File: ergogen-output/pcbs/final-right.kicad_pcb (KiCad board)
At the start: 2 copper layers, 161.7 x 120.6 mm, 61 parts

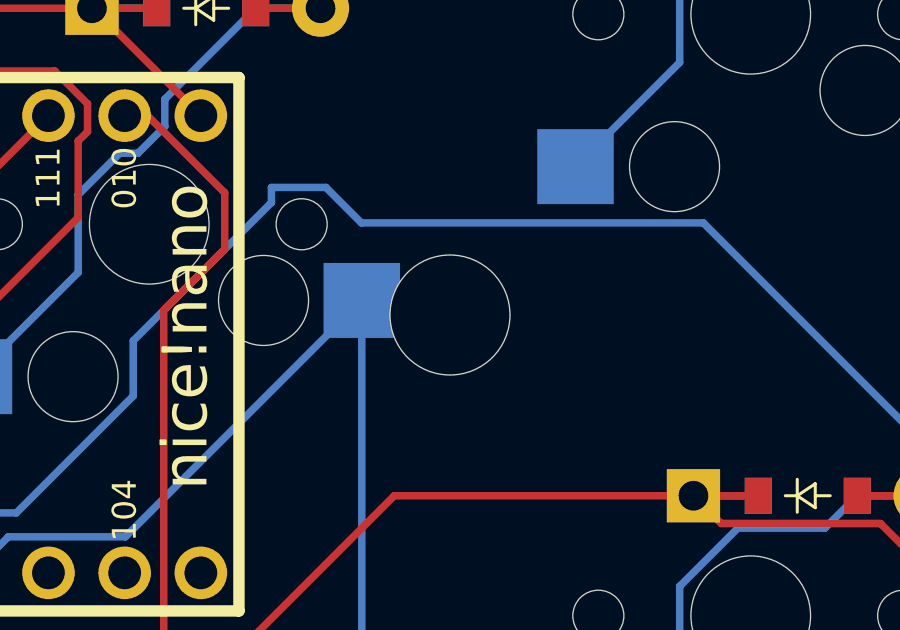
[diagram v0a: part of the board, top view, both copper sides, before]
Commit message: fix pcbs :(
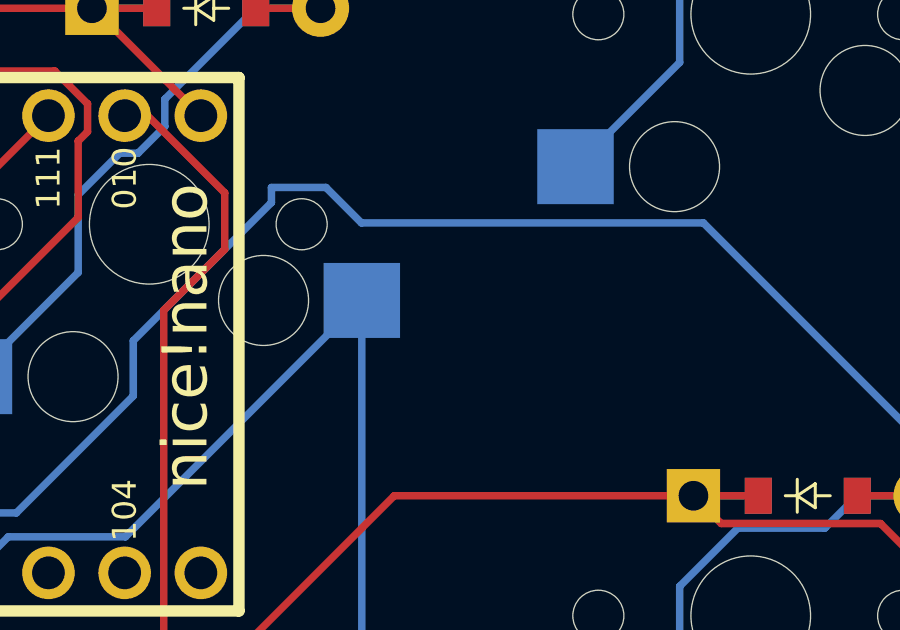
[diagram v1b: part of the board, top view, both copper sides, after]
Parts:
- removed the ? at (300.6, 86.9)
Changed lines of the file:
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@@
 		)
 	)
-	(footprint "HOLE_M2_TH"
-		(layer "F.Cu")
-		(at 300.625 86.875)
-		(property "Reference" ""
-			(at 0 0 0)
-			(layer "F.SilkS")
-			(effects
-				(font
-					(size 1.27 1.27)
-					(thickness 0.15)
-				)
-			)
-		)
-		(property "Value" ""
-			(at 0 0 0)
-			(layer "F.Fab")
-			(effects
-				(font
-					(size 1.27 1.27)
-					(thickness 0.15)
-				)
-			)
-		)
-		(property "Footprint" ""
-			(at 0 0 0)
-			(layer "F.Fab")
-			(hide yes)
-			(effects
-				(font
-					(size 1.27 1.27)
-					(thickness 0.15)
-				)
-			)
-		)
-		(property "Datasheet" ""
-			(at 0 0 0)
-			(layer "F.Fab")
-			(hide yes)
-			(effects
-				(font
-					(size 1.27 1.27)
-					(thickness 0.15)
-				)
-			)
-		)
-		(property "Description" ""
-			(at 0 0 0)
-			(layer "F.Fab")
-			(hide yes)
-			(effects
-				(font
-					(size 1.27 1.27)
-					(thickness 0.15)
-				)
-			)
-		)
-		(attr through_hole)
-		(pad "" np_thru_hole circle
-			(at 0 0 90)
-			(size 4 4)
-			(drill 4)
-			(layers "*.Cu" "*.Mask" "F.SilkS")
-			(clearance 0.3)
-		)
-	)
 	(footprint "ComboDiode"
 		(layer "F.Cu")
@@
 		(layer "Edge.Cuts")
 	)
-	(gr_line
-		(start 362.775 77.825)
-		(end 362.775 77.825)
-		(stroke
-			(width 0.15)
-			(type solid)
-		)
-		(layer "Edge.Cuts")
-	)
 	(gr_arc
 		(start 234.115912 185.296269)
@@
 		(stroke
 			(width 0.15)
-			(type solid)
-		)
-		(layer "Edge.Cuts")
-	)
-	(gr_line
-		(start 358.775 162.025)
-		(end 358.775 162.025)
-		(stroke
-			(width 0.15)

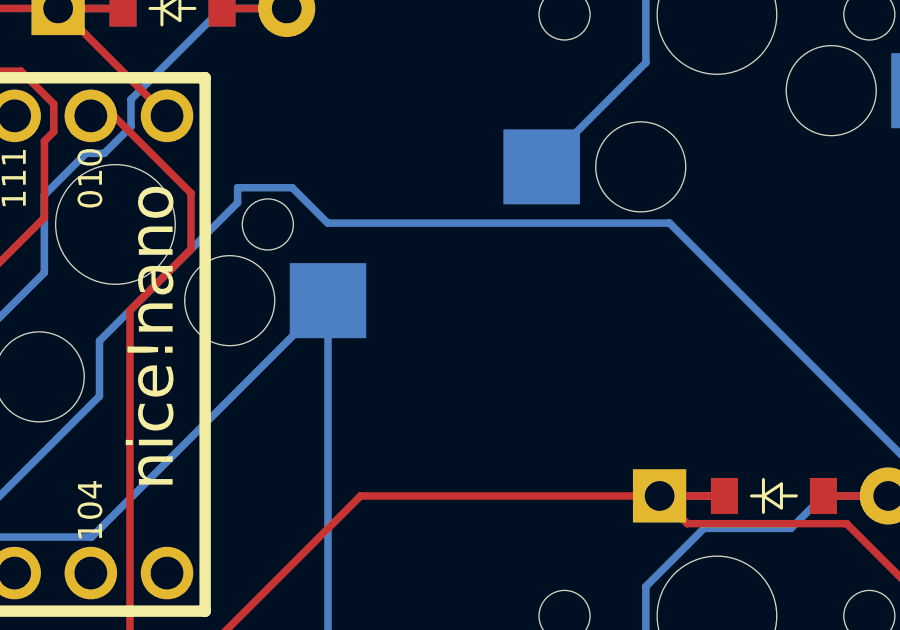
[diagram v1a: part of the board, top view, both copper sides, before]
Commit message: fix pcbs part 2
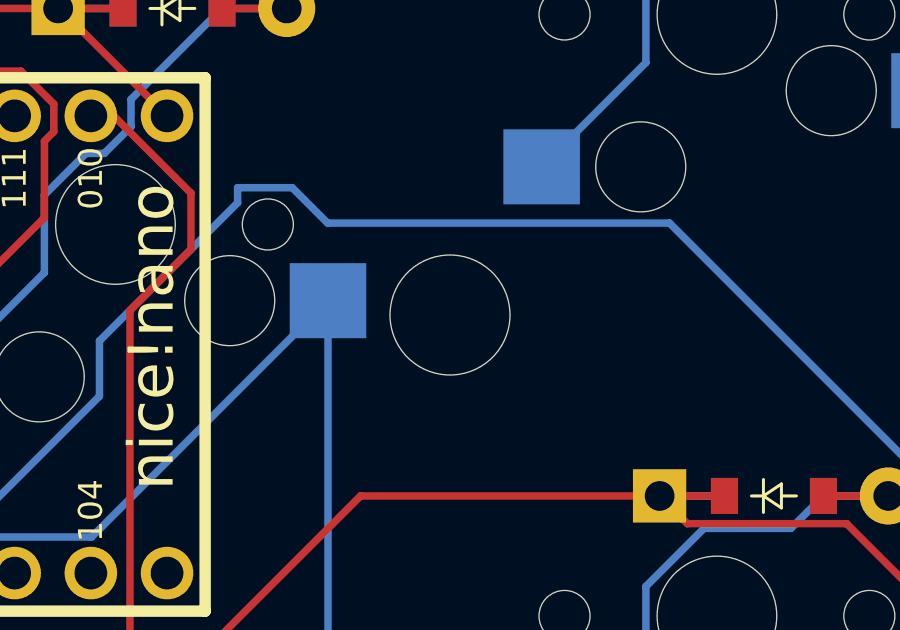
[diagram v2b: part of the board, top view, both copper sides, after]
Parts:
- added ?: , HOLE_M2_TH, F.Cu at (301.8, 86.9)
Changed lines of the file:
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@@
+		)
+	)
+	(footprint "HOLE_M2_TH"
+		(layer "F.Cu")
+		(at 301.752 86.868)
+		(property "Reference" ""
+			(at 0 0 0)
+			(layer "F.SilkS")
+			(effects
+				(font
+					(size 1.27 1.27)
+					(thickness 0.15)
+				)
+			)
+		)
+		(property "Value" ""
+			(at 0 0 0)
+			(layer "F.Fab")
+			(effects
+				(font
+					(size 1.27 1.27)
+					(thickness 0.15)
+				)
+			)
+		)
+		(property "Footprint" ""
+			(at 0 0 0)
+			(layer "F.Fab")
+			(hide yes)
+			(effects
+				(font
+					(size 1.27 1.27)
+					(thickness 0.15)
+				)
+			)
+		)
+		(property "Datasheet" ""
+			(at 0 0 0)
+			(layer "F.Fab")
+			(hide yes)
+			(effects
+				(font
+					(size 1.27 1.27)
+					(thickness 0.15)
+				)
+			)
+		)
+		(property "Description" ""
+			(at 0 0 0)
+			(layer "F.Fab")
+			(hide yes)
+			(effects
+				(font
+					(size 1.27 1.27)
+					(thickness 0.15)
+				)
+			)
+		)
+		(attr through_hole)
+		(pad "" np_thru_hole circle
+			(at 0 0 90)
+			(size 4 4)
+			(drill 4)
+			(layers "F&B.Cu" "*.Mask" "F.SilkS")
+			(clearance 0.3)
 		)
 	)

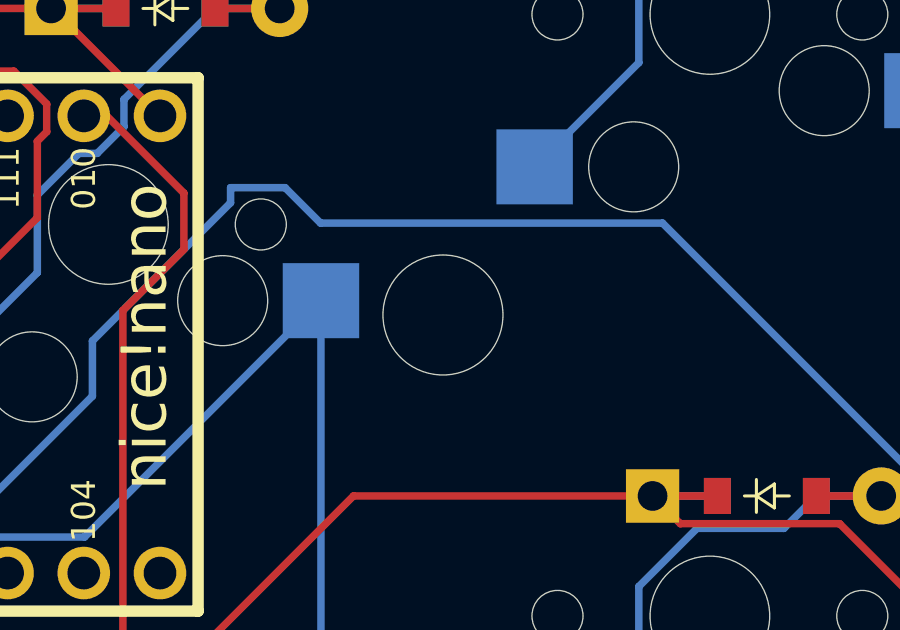
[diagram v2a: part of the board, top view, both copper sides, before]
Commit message: Fix up PCB one last time
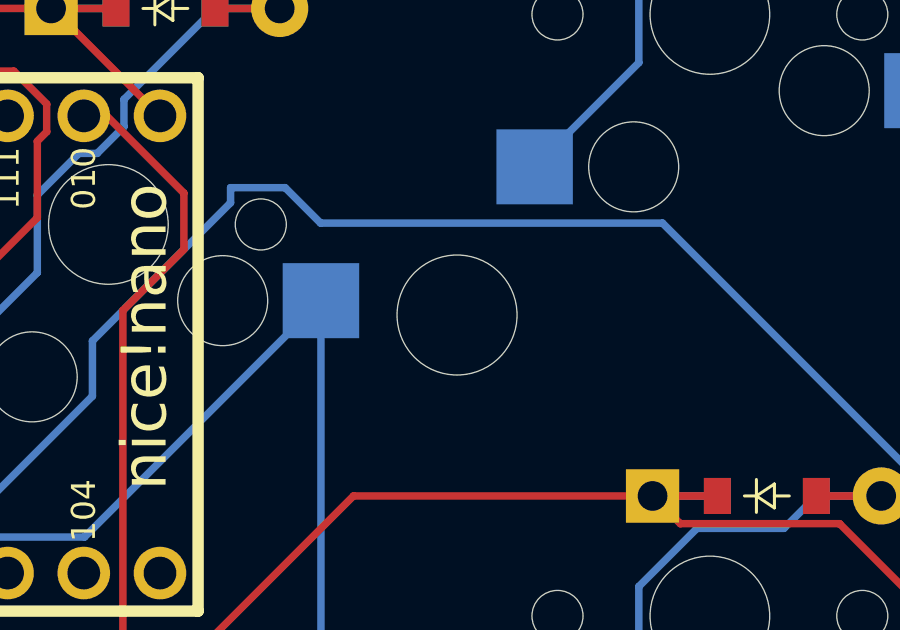
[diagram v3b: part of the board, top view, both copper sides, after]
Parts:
- moved ? 0.47 mm to (302.2, 86.9)
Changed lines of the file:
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@@
 	(footprint "HOLE_M2_TH"
 		(layer "F.Cu")
-		(at 301.752 86.868)
+		(at 302.22182 86.868593)
 		(property "Reference" ""
 			(at 0 0 0)
